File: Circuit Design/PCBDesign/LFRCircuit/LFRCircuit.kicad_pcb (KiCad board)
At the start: 2 copper layers, 74.5 x 60 mm, 30 parts, among them M1 Motor_DC, M2 Motor_DC, U1 L293D, U2 TPS54202DDC

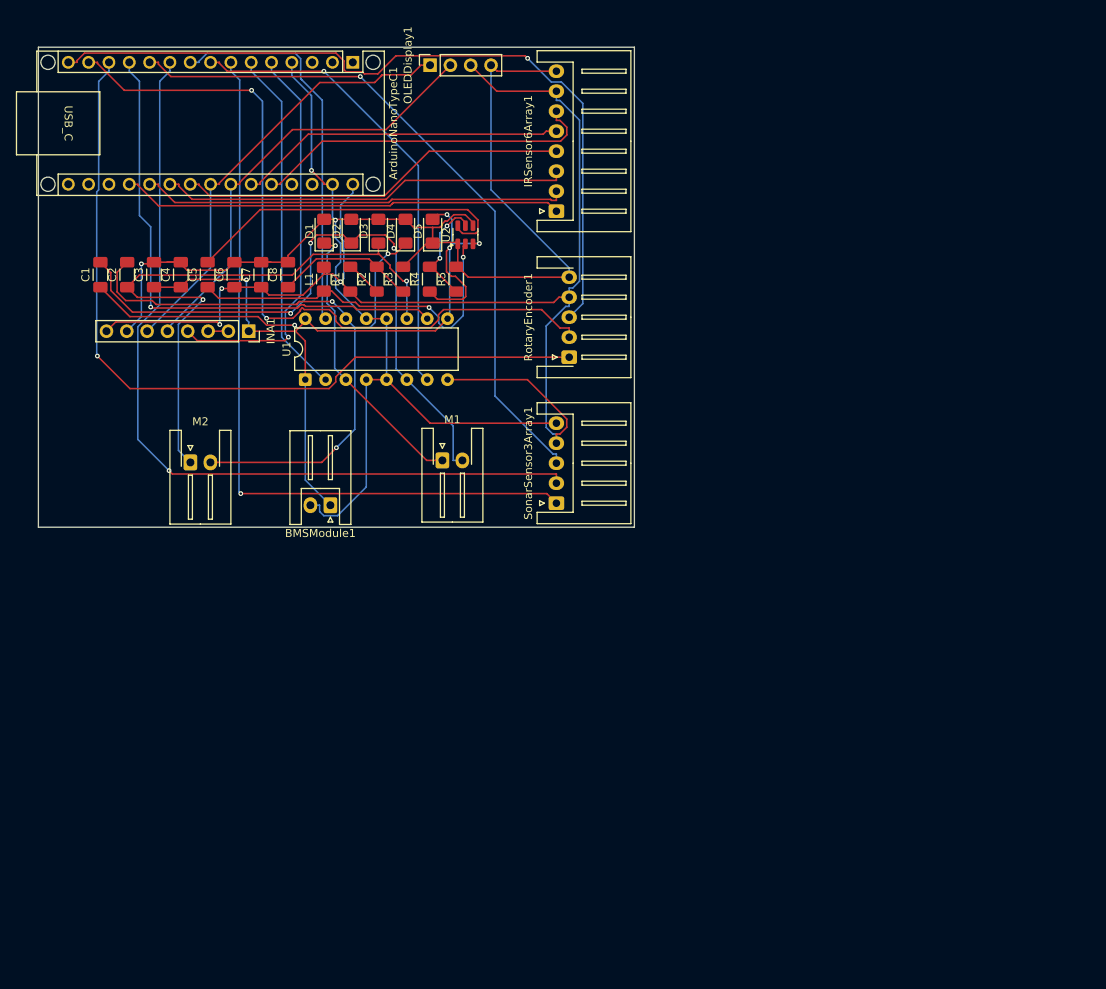
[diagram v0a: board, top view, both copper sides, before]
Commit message: Circuit design is completed
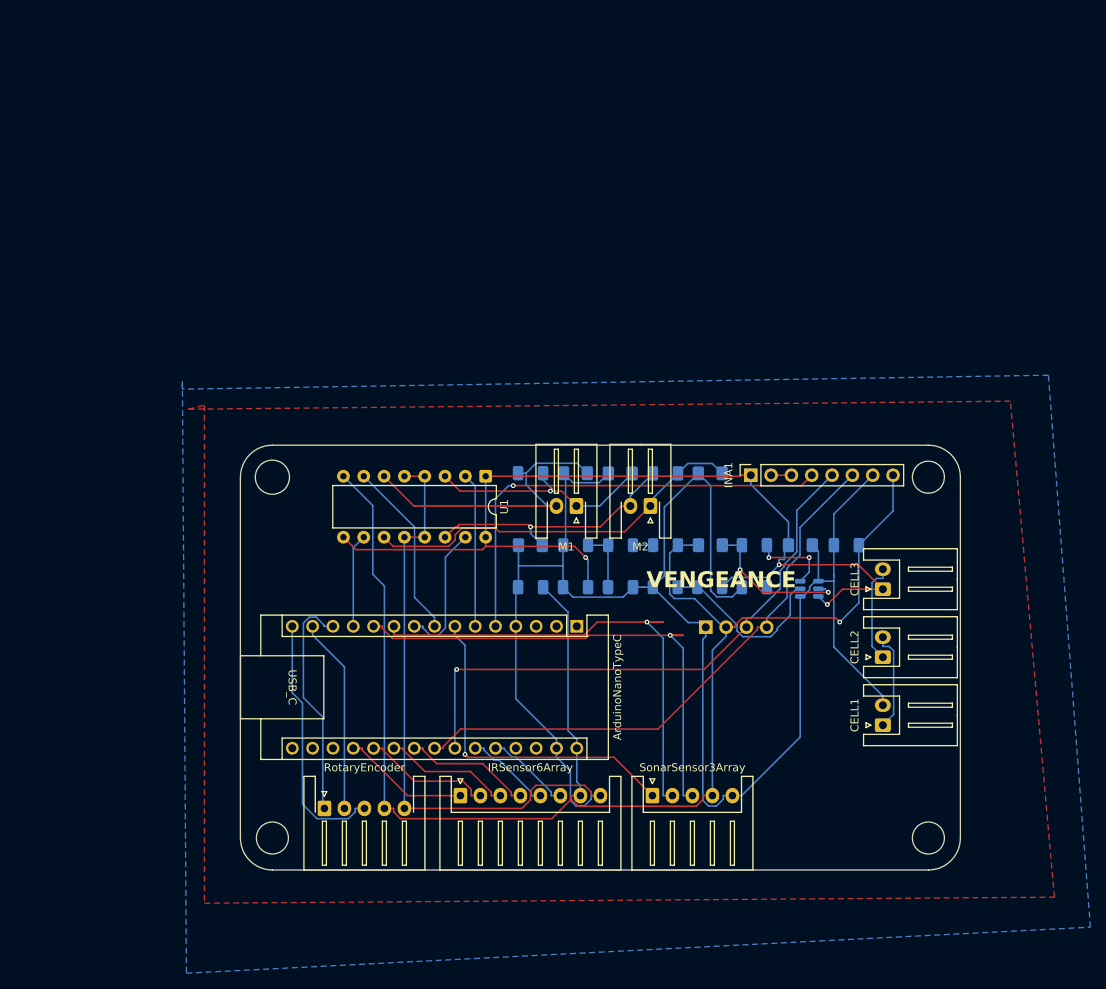
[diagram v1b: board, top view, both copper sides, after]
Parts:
- removed ArduinoNanoTypeC1: ~, ArduinoNano:ArduinoNanoTypeC
- removed BMSModule1: ~, Connector_JST:JST_XH_S2B-XH-A_1x02_P2.50mm_Horizontal
- removed IRSensor6Array1: ~, Connector_JST:JST_XH_S8B-XH-A_1x08_P2.50mm_Horizontal
- removed OLEDDisplay1: ~, Connector_PinSocket_2.54mm:PinSocket_1x04_P2.54mm_Vertical
- removed RotaryEncoder1: ~, Connector_JST:JST_XH_S5B-XH-A-1_1x05_P2.50mm_Horizontal
- removed SonarSensor3Array1: ~, Connector_JST:JST_XH_S5B-XH-A_1x05_P2.50mm_Horizontal
- added ArduinoNanoTypeC: ~, ArduinoNano:ArduinoNanoTypeC, F.Cu at (167.6, 97.1)
- added CELL1: Battery_Cell, Connector_JST:JST_XH_S2B-XH-A_1x02_P2.50mm_Horizontal, F.Cu at (205.8, 109.5)
- added CELL2: Battery_Cell, Connector_JST:JST_XH_S2B-XH-A_1x02_P2.50mm_Horizontal, F.Cu at (205.8, 101.0)
- added CELL3: Battery_Cell, Connector_JST:JST_XH_S2B-XH-A_1x02_P2.50mm_Horizontal, F.Cu at (205.8, 92.5)
- added IRSensor6Array: ~, Connector_JST:JST_XH_S8B-XH-A_1x08_P2.50mm_Horizontal, F.Cu at (153.0, 118.3)
- added J1: OLED_128x64, ScottoKeebs_Components:OLED_128x64, F.Cu at (187.5, 97.2)
- added RotaryEncoder: ~, Connector_JST:JST_XH_S5B-XH-A-1_1x05_P2.50mm_Horizontal, F.Cu at (136.0, 119.9)
- added SonarSensor3Array: ~, Connector_JST:JST_XH_S5B-XH-A_1x05_P2.50mm_Horizontal, F.Cu at (177.0, 118.3)
- C1, C2, C3, C4, C5, C6, C7, C8, D1, D2, D3, D4, D5, L1, R1, R2, R3, R4, R5, U2: moved to B.Cu
- moved C4 81.7 mm to (189.8, 92.2), turned to 180 degrees
- moved C7 80.6 mm to (201.2, 87.0), turned to 180 degrees
- moved C5 76.3 mm to (189.8, 87.0), turned to 0 degrees
- moved C2 71.7 mm to (178.6, 78.0), turned to 180 degrees
- moved C3 65.6 mm to (167.4, 92.2), turned to 180 degrees
- moved INA1 65.3 mm to (189.3, 78.2), turned to 90 degrees
- moved U2 61.7 mm to (196.6, 92.5), turned to 180 degrees
- moved D5 60.4 mm to (195.5, 87.0), turned to 180 degrees
- moved C1 59.2 mm to (161.8, 78.0), turned to 180 degrees
- moved L1 58.7 mm to (184.2, 87.0), turned to 180 degrees
- moved M2 57.8 mm to (176.8, 82.1), turned to 180 degrees
- moved C8 57.0 mm to (173.0, 92.2), turned to 0 degrees
- moved C6 53.8 mm to (161.8, 92.2), turned to 180 degrees
- moved R4 52.0 mm to (184.2, 92.2), turned to 180 degrees
- moved R1 51.6 mm to (178.6, 87.0), turned to 180 degrees
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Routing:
- net GND: track 222.7 -> 297.0 mm, vias 3 -> 0
- net /RE_CLK: track 100.0 -> 28.8 mm, vias 1 -> 0
- net /RE_DT: track 94.4 -> 24.4 mm, vias 2 -> 0
- net /RE_SW: track 97.5 -> 32.0 mm, vias 1 -> 0
- net /M2B: track 67.4 -> 11.7 mm, vias 1 -> 0
- net Net-(D4-K): track 83.9 -> 33.4 mm, vias 3 -> 1
- net /S1: track 94.4 -> 44.1 mm
- net Net-(D2-K): track 81.1 -> 39.1 mm, vias 3 -> 0
- net /IR1: track 55.4 -> 16.0 mm
- net /S2: track 104.1 -> 65.2 mm
- net /IR2: track 53.5 -> 16.3 mm
- net Net-(D1-K): track 67.3 -> 30.1 mm, vias 2 -> 1
- net /M1B: track 58.6 -> 22.4 mm, vias 1 -> 0
- net /IR3: track 51.4 -> 16.1 mm
- net /IR4: track 48.8 -> 16.1 mm
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- added copper zone on F.Cu, net +12V
- added copper zone on B.Cu, net GND
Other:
- board size 74.5 x 60 mm -> 90 x 53.1 mm
- board text added: "VENGEANCE"
